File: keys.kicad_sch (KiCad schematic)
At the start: 7 parts, among them SW1 RotaryEncoder_Switch

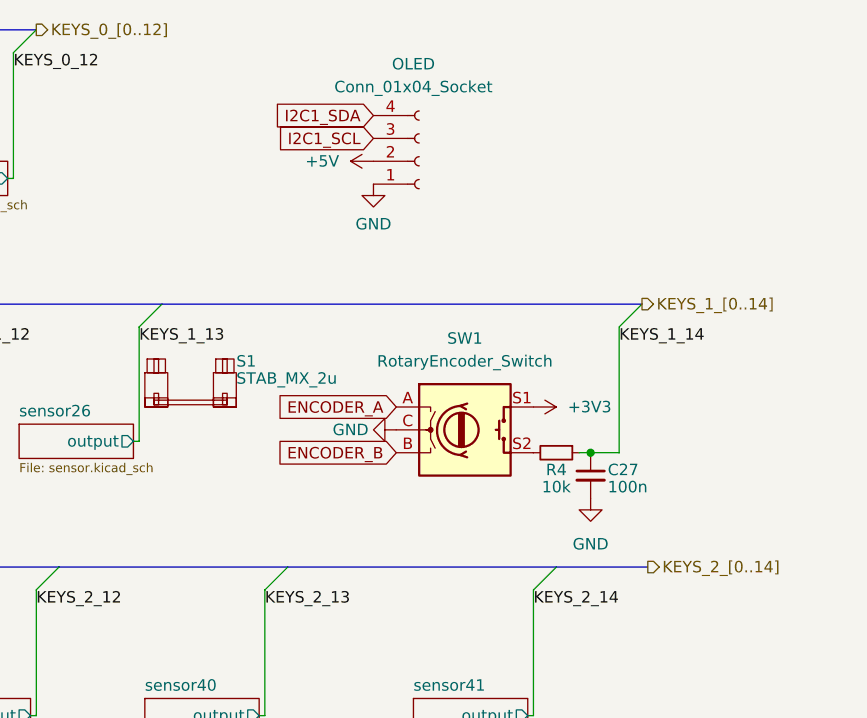
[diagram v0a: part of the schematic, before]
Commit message: finish routing
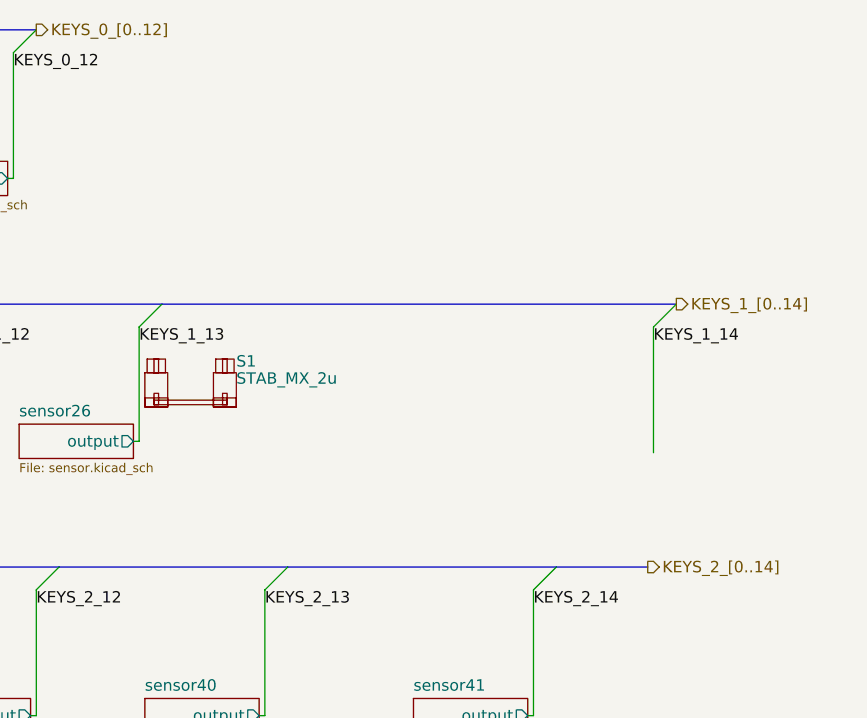
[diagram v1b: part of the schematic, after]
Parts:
- removed C27: 100n, Capacitor_SMD:C_0402_1005Metric, symbol Device:C_Small
- removed OLED: Conn_01x04_Socket, MoonBoard:OLED Module, symbol Connector:Conn_01x04_Socket
- removed R4: 10k, Resistor_SMD:R_0402_1005Metric, symbol Device:R_Small
- removed SW1: RotaryEncoder_Switch, PCM_marbastlib-various:ROT_Alps_EC11E-Switch, symbol Device:RotaryEncoder_Switch
